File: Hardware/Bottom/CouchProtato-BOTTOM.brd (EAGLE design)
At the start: 33 x 33 mm, 32 parts, among them U1 AD5242-SO16

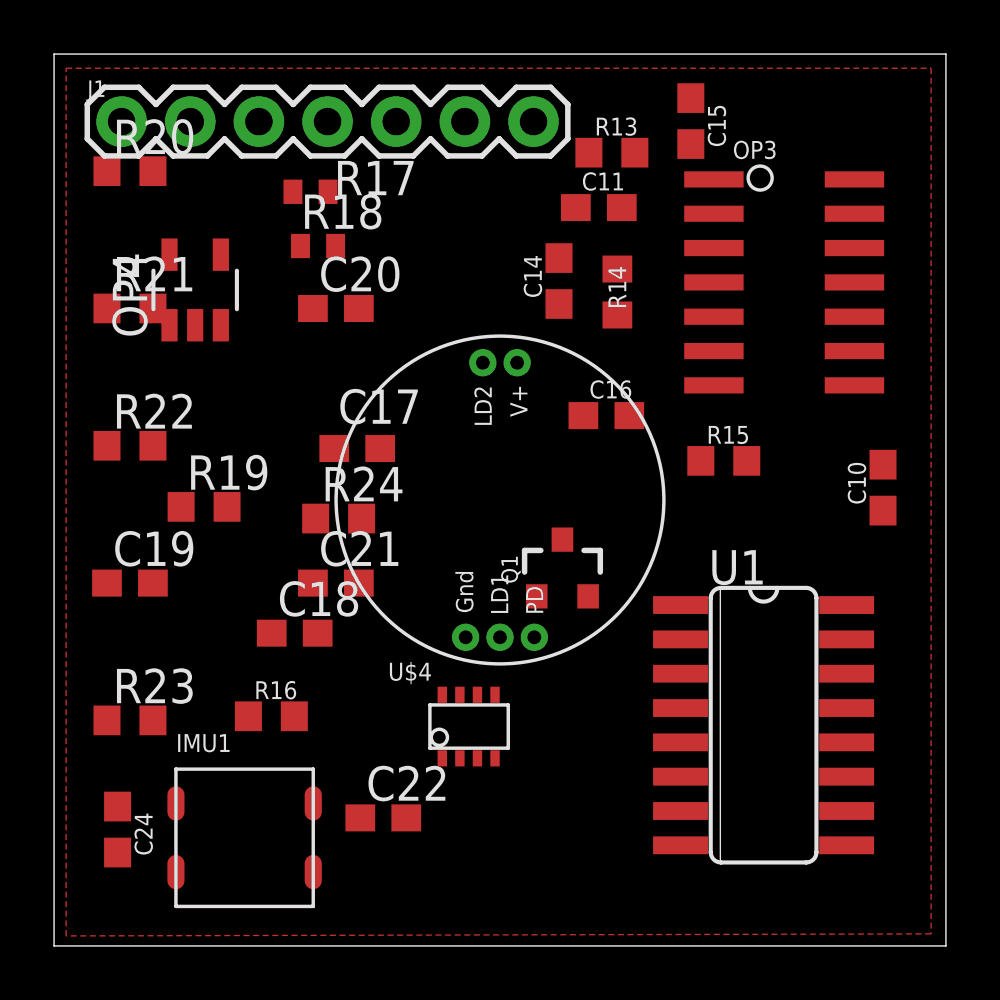
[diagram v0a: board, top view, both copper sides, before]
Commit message: Progress on routing bottom board and schematic
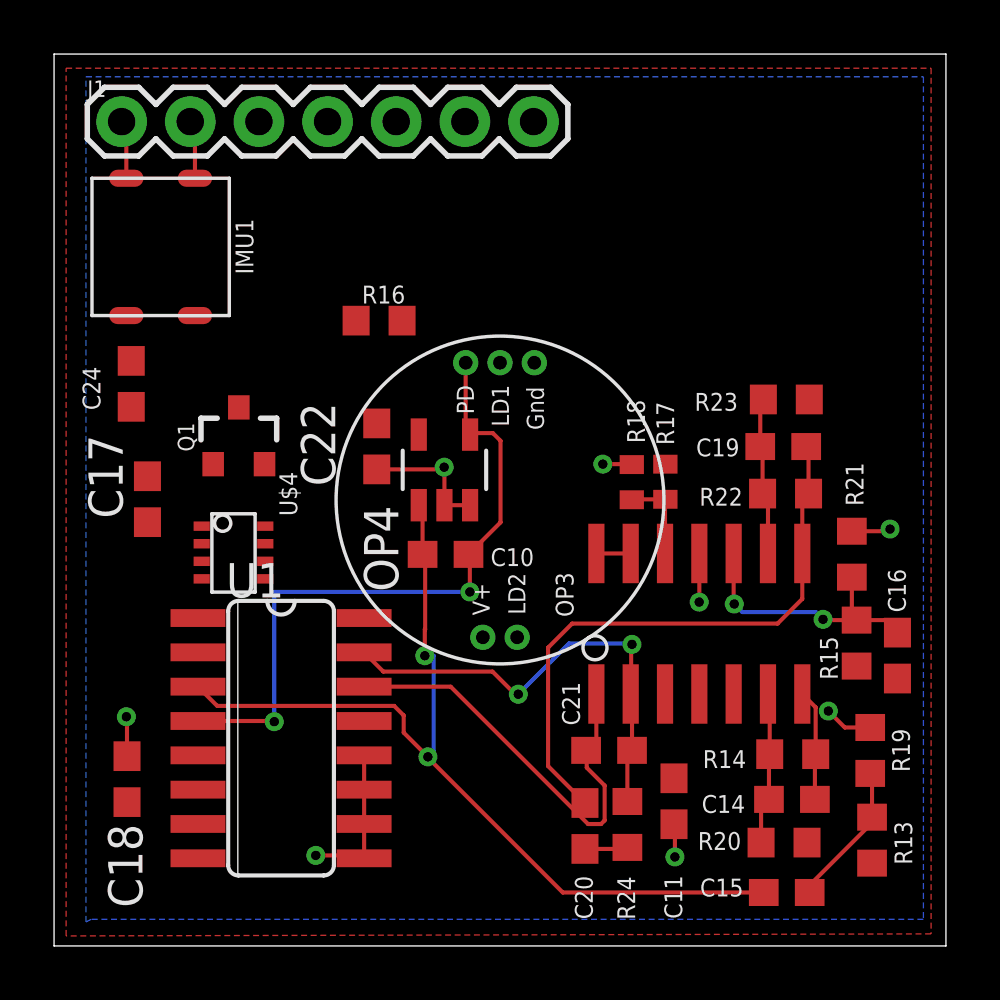
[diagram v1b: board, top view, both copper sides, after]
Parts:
- moved R20 34.7 mm to (29.5, 6.32), turned to 180 degrees
- moved C15 28.8 mm to (29.6, 4.48), turned to 0 degrees
- moved R21 28.2 mm to (32.0, 17.0), turned to 270 degrees
- moved R13 27.2 mm to (32.8, 6.41), turned to 270 degrees
- moved R23 27.0 mm to (29.6, 22.7), turned to 180 degrees
- moved R19 26.2 mm to (32.7, 9.73), turned to 270 degrees
- moved C19 24.7 mm to (29.5, 21.0), turned to 180 degrees
- moved R22 24.3 mm to (29.6, 19.2)
- moved C11 22.1 mm to (25.4, 7.85), turned to 90 degrees
- moved IMU1 22.1 mm to (6.44, 28.4), turned to 90 degrees
- moved C20 21.2 mm to (22.1, 6.94), turned to 270 degrees
- moved C14 21.0 mm to (29.8, 7.92), turned to 180 degrees
- moved R14 18.3 mm to (29.8, 9.60), turned to 0 degrees
- moved U1 17.9 mm to (10.9, 10.2)
- moved R17 17.0 mm to (25.1, 19.7), turned to 90 degrees
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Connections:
- removed net LED: Q1.3
- net 3.3V: now also J1.4
- net GND: now also J1.3
- net LED.C: now also Q1.3
- net SCL: now also J1.2
- net SDA: now also J1.1
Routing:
- net A6/TIA: track 0.00 -> 34.3 mm, vias 0 -> 2
- net PD.C: track 0.00 -> 25.0 mm, vias 0 -> 2
- net N$19: track 0.00 -> 22.2 mm
- net GND: track 0.00 -> 19.4 mm, vias 0 -> 8
- net G.W2: track 0.00 -> 17.6 mm, vias 0 -> 2
- net A7/PPG: track 0.00 -> 16.2 mm
- net N$17: track 0.00 -> 10.0 mm, vias 0 -> 2
- net N$18: track 0.00 -> 5.86 mm
- net N$15: track 0.00 -> 5.78 mm
- net N$13: track 0.00 -> 5.39 mm
- net N$16: track 0.00 -> 4.12 mm
- net N$10: track 0.00 -> 3.27 mm
- net SDA: track 0.00 -> 2.17 mm
- net SCL: track 0.00 -> 2.17 mm
- net N$20: track 0.00 -> 1.59 mm
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- added copper zone on layer 16, net GND
